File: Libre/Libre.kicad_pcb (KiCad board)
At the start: 2 copper layers, 43.8 x 91.8 mm, 20 parts, among them J1 4.2inch E-Ink Display Module, J2 Micro_SD_Card, J3 Battery connector, SW1 UP, SW2 DOWN, SW3 PREVOUS, SW4 NEXT, SW5 HOME, SW6 SW_SPDT, U1 ESP32-S3-DEVKITC-1-N16R8, U2 MCP73831-2-OT, U3 AP2112K-3.3

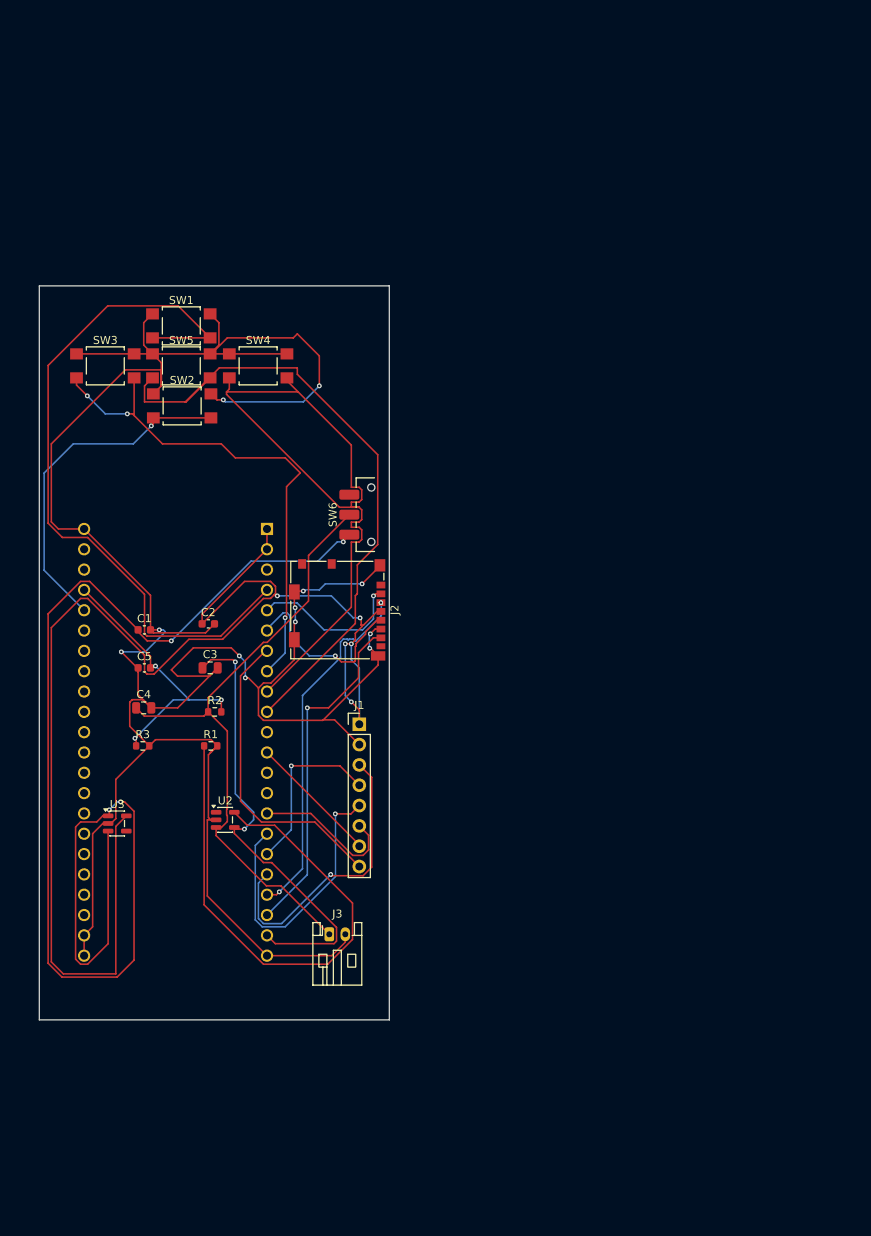
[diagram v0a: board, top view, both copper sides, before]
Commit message: CAD Change
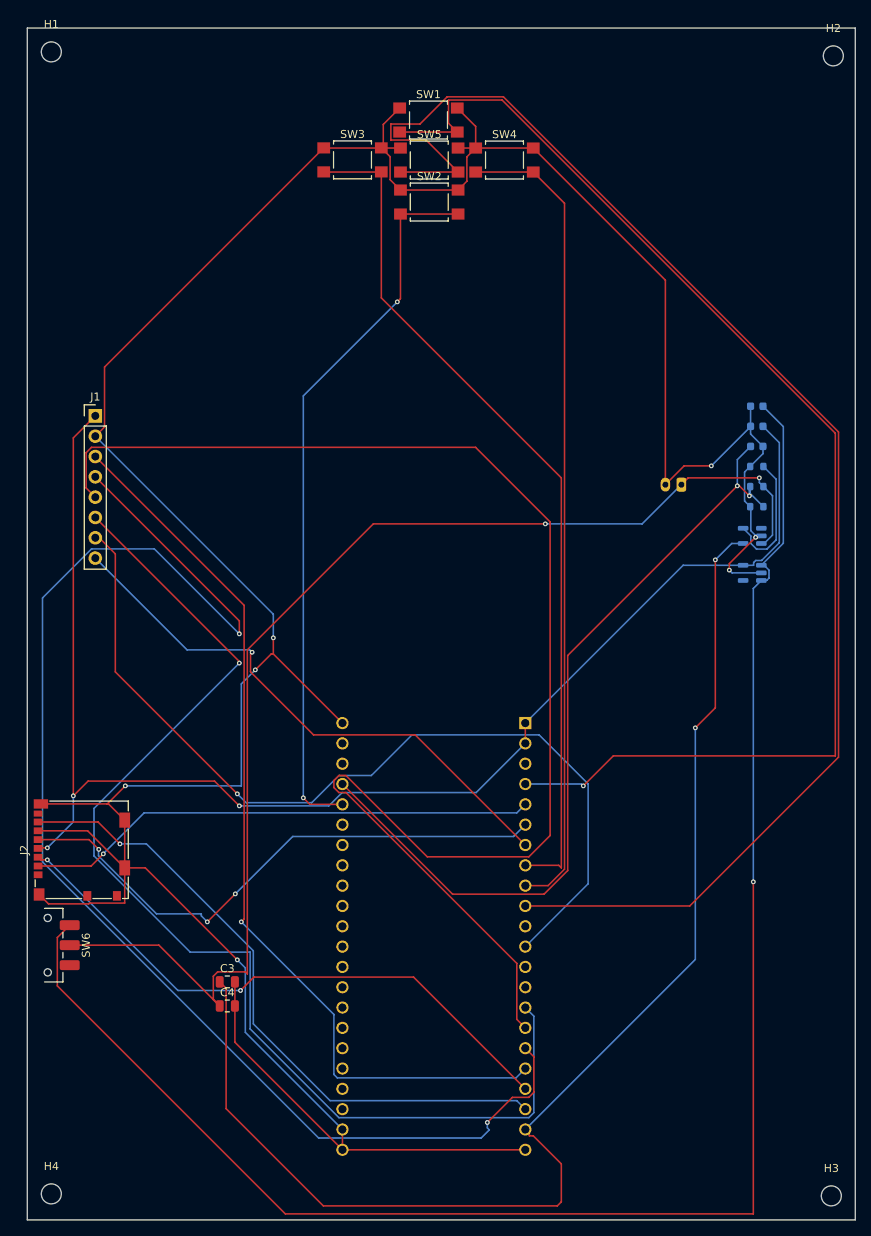
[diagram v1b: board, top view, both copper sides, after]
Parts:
- added H1: MountingHole, MountingHole:MountingHole_2.5mm, F.Cu at (102.8, 24.8)
- added H2: MountingHole, MountingHole:MountingHole_2.5mm, F.Cu at (200.5, 25.2)
- added H3: MountingHole, MountingHole:MountingHole_2.5mm, F.Cu at (200.2, 167.8)
- added H4: MountingHole, MountingHole:MountingHole_2.5mm, F.Cu at (102.8, 167.5)
- C1, C2, C5, J3, R1, R2, R3, U2, U3: moved to B.Cu
- moved U3 85.3 mm to (190.4, 89.9), turned to 180 degrees
- moved R3 82.4 mm to (190.9, 81.6), turned to 180 degrees
- moved C1 81.5 mm to (190.9, 69.0), turned to 180 degrees
- moved C5 81.4 mm to (190.9, 74.1), turned to 180 degrees
- moved R1 76.7 mm to (190.9, 76.6), turned to 180 degrees
- moved U2 74.8 mm to (190.4, 85.2), turned to 180 degrees
- moved R2 73.4 mm to (190.9, 79.1), turned to 180 degrees
- moved C2 72.9 mm to (190.9, 71.6), turned to 180 degrees
- moved J3 71.4 mm to (181.5, 78.8), turned to 180 degrees
- moved SW6 67.3 mm to (102.3, 136.4), turned to -90 degrees
- moved J1 50.7 mm to (108.2, 70.2)
- moved J2 43.8 mm to (106.5, 124.5), turned to 90 degrees
- moved U1 40.4 mm to (150.6, 138.6)
- moved SW5 40.3 mm to (150.0, 38.3)
- moved SW3 40.2 mm to (140.4, 38.2)
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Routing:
- net CLK: track 21.8 -> 176.5 mm, vias 1 -> 2
- net CS: track 35.6 -> 181.3 mm, vias 1 -> 0
- net DC: track 18.6 -> 145.3 mm, vias 0 -> 1
- net USB_5V: track 57.7 -> 159.9 mm
- net Net-(U1-GPIO17): track 81.5 -> 181.5 mm
- net RST: track 16.5 -> 113.6 mm, vias 0 -> 1
- net GND: track 339.6 -> 417.8 mm, vias 12 -> 7
- net DIN: track 36.8 -> 114.5 mm
- net +BATT: track 78.6 -> 153.6 mm, vias 0 -> 2
- net Net-(U1-GPIO1): track 35.2 -> 104.0 mm, vias 3 -> 2
- net Net-(U1-GPIO4): track 90.4 -> 158.0 mm, vias 0 -> 1
- net Net-(U2-PROG): track 66.8 -> 16.1 mm
- net SD_CLK: track 22.8 -> 70.9 mm, vias 1 -> 3
- net Net-(U1-GPIO2): track 43.4 -> 90.4 mm, vias 1 -> 2
- net SD_CS: track 19.6 -> 64.1 mm
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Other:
- board size 43.8 x 91.8 mm -> 103.5 x 149 mm
